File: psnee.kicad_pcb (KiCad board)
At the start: 2 copper layers, 21 x 36 mm, 10 parts, among them IC1 ATTINY45, P1 CONN_ICSP

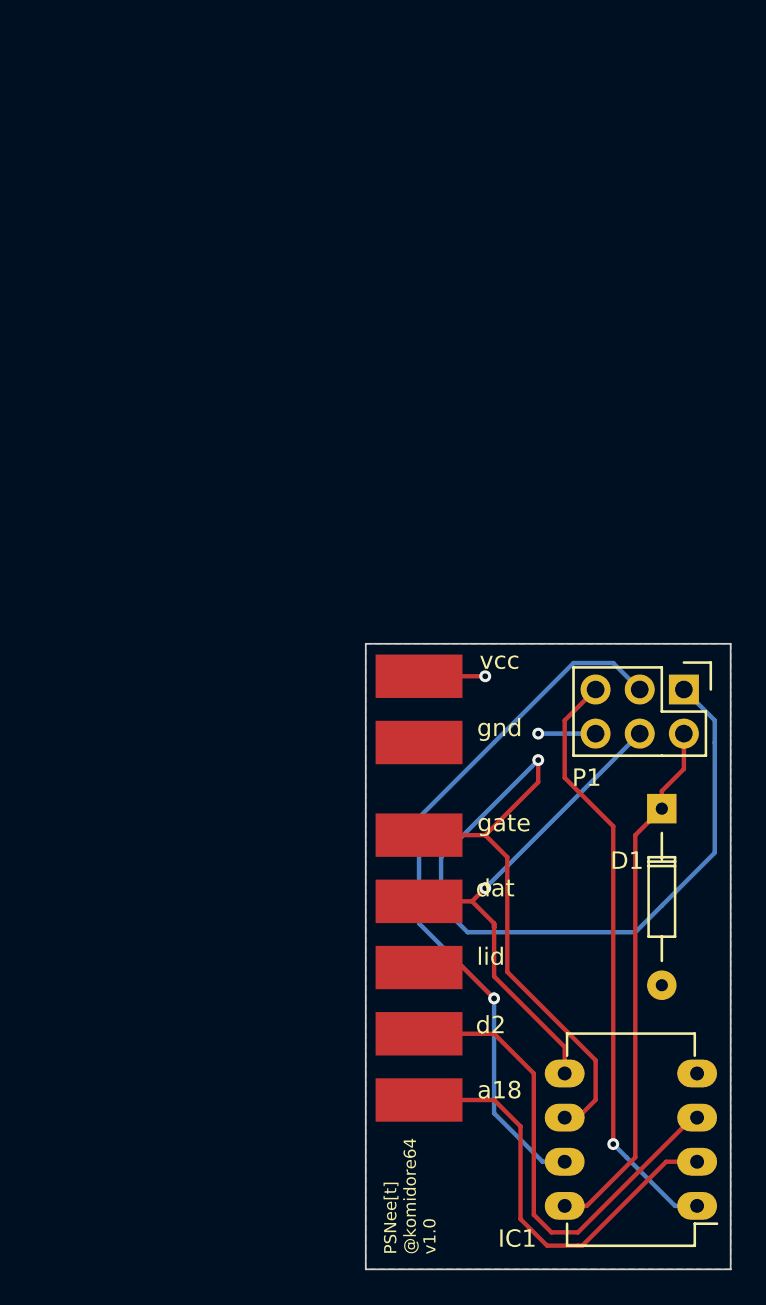
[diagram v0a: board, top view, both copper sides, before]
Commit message: pcb for v2.0
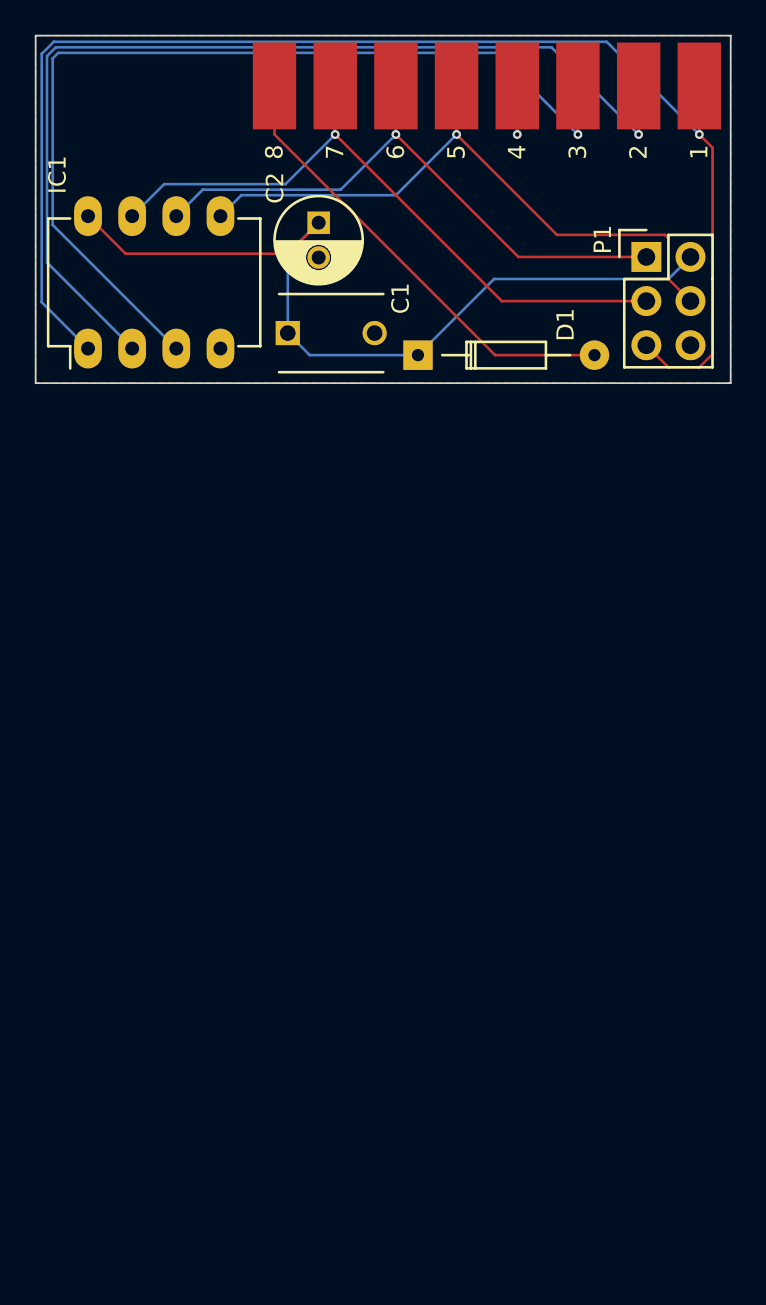
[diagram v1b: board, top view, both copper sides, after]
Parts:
- removed a18, d2, dat, gate, gnd, lid, vcc: wire_pad_2.5_5mm_single, psnee:wire_pad_2.5_5mm_single
- added 1: wire_pad_2.5_5mm_single, psnee:wire_pad_2.5_5mm_single, F.Cu at (163.2, 52.9)
- added 2: wire_pad_2.5_5mm_single, psnee:wire_pad_2.5_5mm_single, F.Cu at (159.7, 52.9)
- added 3: wire_pad_2.5_5mm_single, psnee:wire_pad_2.5_5mm_single, F.Cu at (156.2, 52.9)
- added 4: wire_pad_2.5_5mm_single, psnee:wire_pad_2.5_5mm_single, F.Cu at (152.7, 52.9)
- added 5: wire_pad_2.5_5mm_single, psnee:wire_pad_2.5_5mm_single, F.Cu at (149.2, 52.9)
- added 6: wire_pad_2.5_5mm_single, psnee:wire_pad_2.5_5mm_single, F.Cu at (145.7, 52.9)
- added 7: wire_pad_2.5_5mm_single, psnee:wire_pad_2.5_5mm_single, F.Cu at (142.2, 52.9)
- added 8: wire_pad_2.5_5mm_single, psnee:wire_pad_2.5_5mm_single, F.Cu at (138.7, 52.9)
- added C1: 100nF, Capacitors_ThroughHole:C_Disc_D6_P5, F.Cu at (139.5, 67.1)
- added C2: 100uF, Capacitors_ThroughHole:C_Radial_D5_L11_P2, F.Cu at (141.3, 60.8)
- IC1: value ATTINY45 -> attiny45
- P1: value CONN_ICSP -> header
- moved IC1 60.5 mm to (128.0, 68.0), turned to 90 degrees
- moved D1 29.6 mm to (147.0, 68.4), turned to 0 degrees
- moved P1 25.0 mm to (160.1, 62.7), turned to 0 degrees
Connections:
- net /data renamed /5
- net /gate renamed /6
- net /lid renamed /7
- net Net-(IC1-Pad1) renamed /1
- IC1 pad 2: /biosA18 -> /2
- IC1 pad 3: /biosD2 -> /3
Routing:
- net /2: track 0.00 -> 58.0 mm, vias 0 -> 1
- net /3: track 0.00 -> 54.7 mm, vias 0 -> 1
- net /1: track 34.4 -> 78.8 mm
- net /6: track 68.6 -> 34.7 mm
- net /biosD2: track 28.2 -> 0.00 mm
- net /biosA18: track 24.6 -> 0.00 mm
- net VCC: track 3.81 -> 26.5 mm, vias 1 -> 0
- net Net-(C1-Pad1): track 30.8 -> 48.0 mm
- net /7: track 46.6 -> 38.3 mm
- net /5: track 29.6 -> 37.1 mm
- net GND: track 3.30 -> 2.79 mm
- added copper zone on B.Cu, net GND
- removed copper zone on B.Cu, net VCC
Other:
- board size 21 x 36 mm -> 40 x 20 mm
- net class Default: clearance 0.254 -> 0.1524; trace_width 0.254 -> 0.1524; via_dia 0.6858 -> 0.508; via_drill 0.3302 -> 0.254
- rule trace_clearance: 0.254 -> 0.1524
- rule via_min_drill: 0.3302 -> 0.254
- rule via_min_size: 0.6858 -> 0.4
- board text removed: "PSNee[t] @komidore64 v1.0"
